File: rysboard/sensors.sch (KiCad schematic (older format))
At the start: 11 parts, among them J10 ToF1, J11 ToF2, J12 ToF3, J13 ToF4, J15 ToF5, J16 ToF6, J9 IMU, Q2 DMP2075UFDB, Q7 NST847BDP6T5G

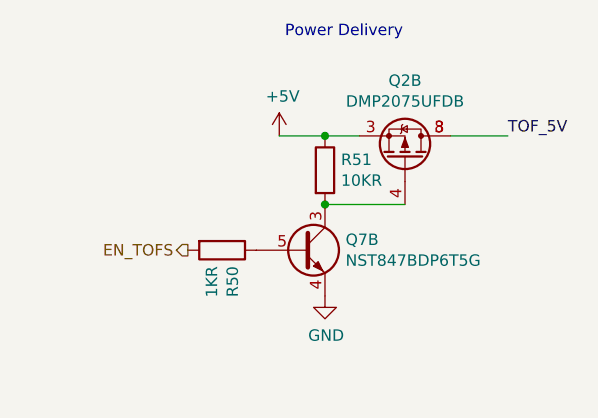
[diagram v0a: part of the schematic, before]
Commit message: Bom finished pcb cleanup started
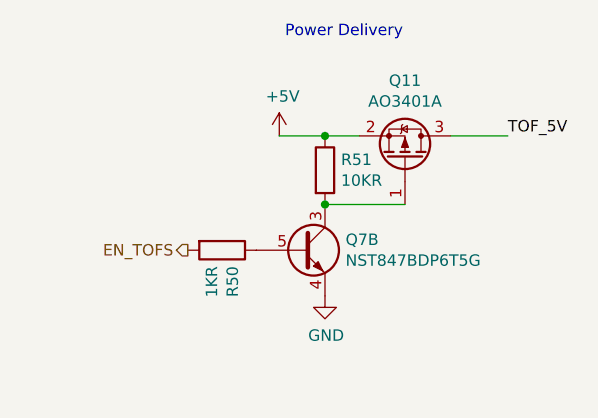
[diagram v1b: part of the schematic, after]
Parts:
- removed Q2: DMP2075UFDB, SamacSys_Parts:DMP2075UFDB7, symbol rysboard:DMP2075UFDB
- added Q11: AO3401A, Package_TO_SOT_SMD:SOT-23, symbol Transistor_FET:AO3401A
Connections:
- net +5V: now also Q11.2 (S)
- net TOF_5V: now also Q11.3 (D)
- net at Q7.3 (C2), R51.2: now also Q11.1 (G)
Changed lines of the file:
@@
 	5700 1250 5450 1250
-$Comp
-L rysboard:DMP2075UFDB Q2
-U 2 1 605EBA08
-P 5250 1350
-F 0 "Q2" V 5592 1350 50  0000 C CNN
-F 1 "DMP2075UFDB" V 5501 1350 50  0000 C CNN
-F 2 "SamacSys_Parts:DMP2075UFDB7" H 5450 1275 50  0001 L CIN
-F 3 "" H 5250 1350 50  0001 L CNN
-	2    5250 1350
-	0    1    -1   0
-$EndComp
 $Comp
 L Device:R R50
@@
 Text Notes 4725 825  0    50   ~ 0
 Power Delivery\n
+$Comp
+L Transistor_FET:AO3401A Q11
+U 1 1 608DDCED
+P 5250 1350
+F 0 "Q11" V 5592 1350 50  0000 C CNN
+F 1 "AO3401A" V 5501 1350 50  0000 C CNN
+F 2 "Package_TO_SOT_SMD:SOT-23" H 5450 1275 50  0001 L CIN
+F 3 "http://www.aosmd.com/pdfs/datasheet/AO3401A.pdf" H 5250 1350 50  0001 L CNN
+	1    5250 1350
+	0    1    -1   0
+$EndComp
 $EndSCHEMATC
